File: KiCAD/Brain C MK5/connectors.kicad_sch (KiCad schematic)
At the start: 9 parts, among them J10 Conn_01x10, J3 Conn_01x06, J4 Conn_01x06, J6 Conn_01x10, J7 Conn_01x10, J8 Conn_01x04, J9 Conn_01x04

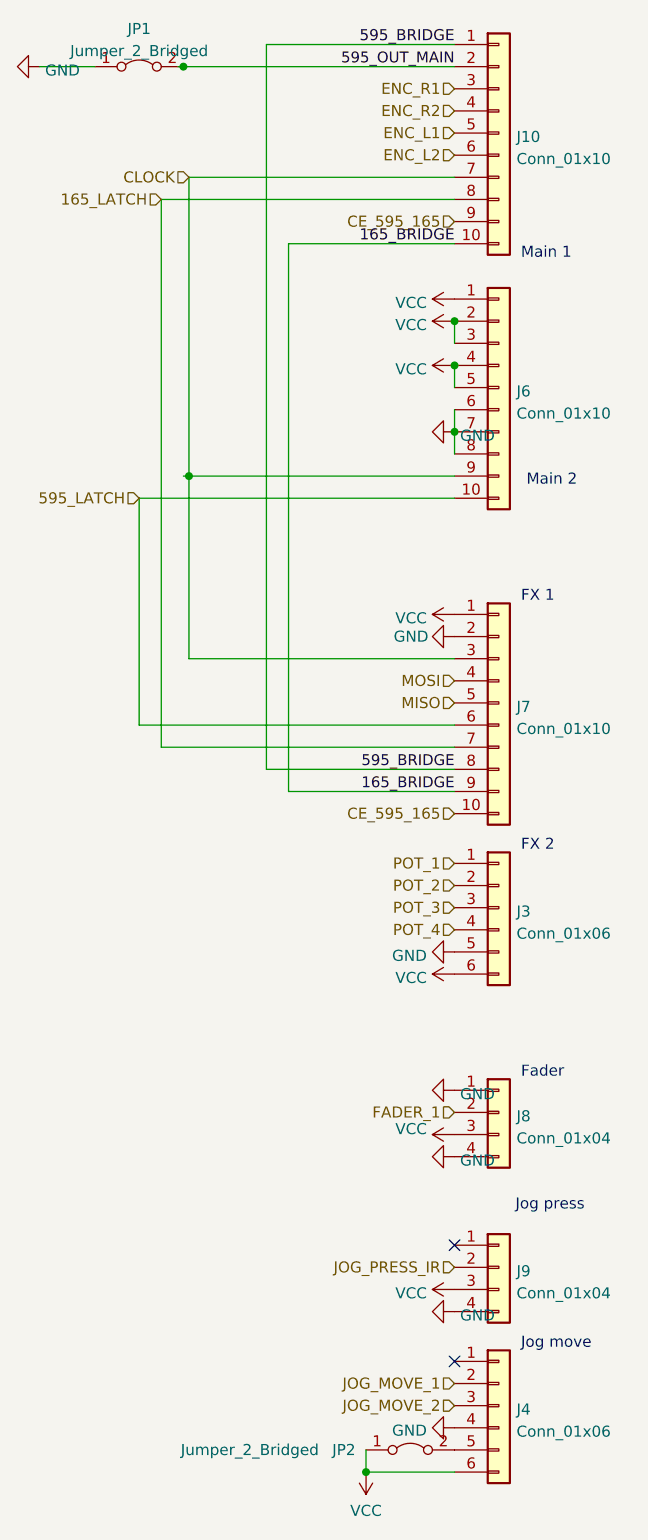
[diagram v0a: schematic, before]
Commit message: work
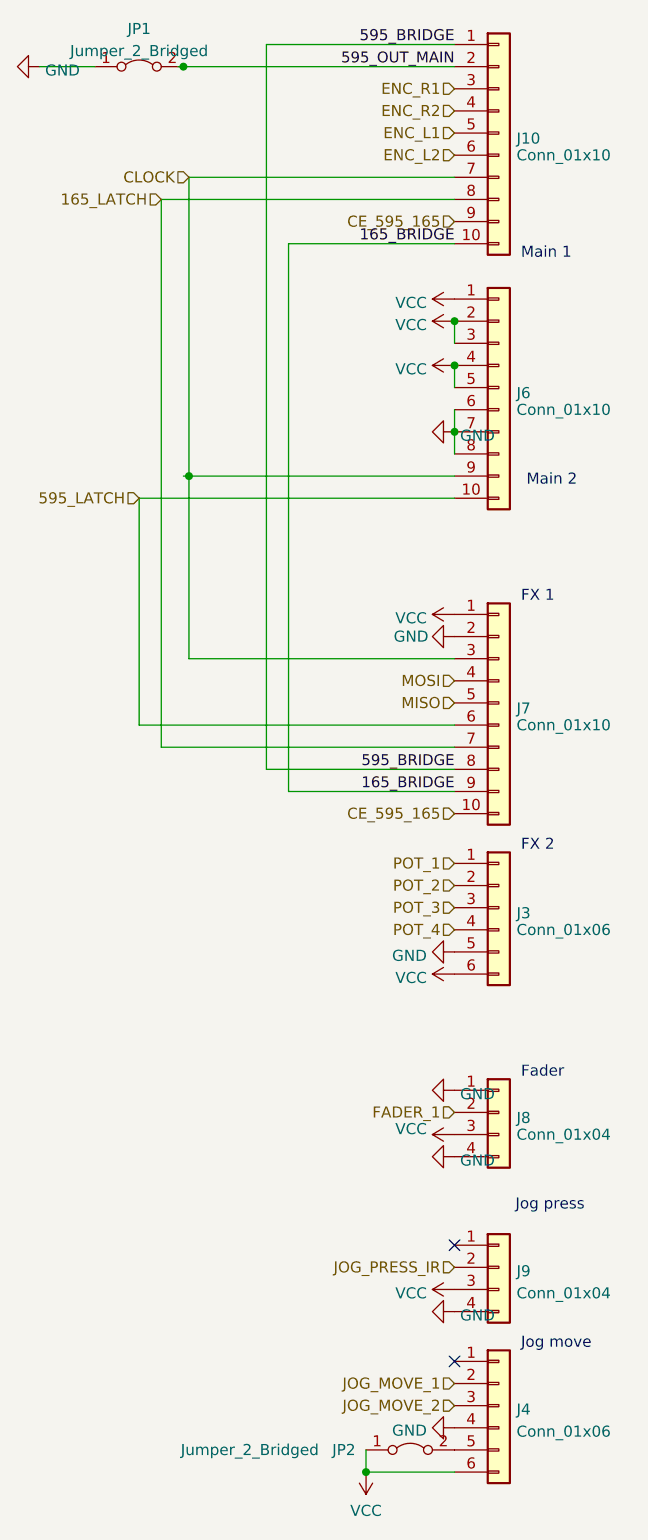
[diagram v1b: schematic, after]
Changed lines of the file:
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@@
   (symbol (lib_id "Connector_Generic:Conn_01x06") (at 278.13 113.03 0) (unit 1)
     (in_bom yes) (on_board yes) (dnp no) (fields_autoplaced)
-    (property "Reference" "J3" (at 280.162 113.4653 0)
-      (effects (font (size 1.27 1.27)) (justify left))
-    )
-    (property "Value" "Conn_01x06" (at 280.162 116.0022 0)
+    (property "Reference" "J3" (at 280.162 113.6563 0)
+      (effects (font (size 1.27 1.27)) (justify left))
+    )
+    (property "Value" "Conn_01x06" (at 280.162 115.5773 0)
       (effects (font (size 1.27 1.27)) (justify left))
     )
@@
         )
         (path "/0b6afff7-70c7-4317-8634-925834fa4d63/1ed31a1a-676b-43f1-be17-fc7627fd91ec"
-          (reference "J3") (unit 1)
+          (reference "J6") (unit 1)
         )
       )
@@
   (symbol (lib_id "Connector_Generic:Conn_01x10") (at 278.13 24.13 0) (unit 1)
     (in_bom yes) (on_board yes) (dnp no) (fields_autoplaced)
-    (property "Reference" "J10" (at 280.162 24.5653 0)
-      (effects (font (size 1.27 1.27)) (justify left))
-    )
-    (property "Value" "Conn_01x10" (at 280.162 27.1022 0)
+    (property "Reference" "J10" (at 280.162 24.7563 0)
+      (effects (font (size 1.27 1.27)) (justify left))
+    )
+    (property "Value" "Conn_01x10" (at 280.162 26.6773 0)
       (effects (font (size 1.27 1.27)) (justify left))
     )
@@
         )
         (path "/0b6afff7-70c7-4317-8634-925834fa4d63/1ed31a1a-676b-43f1-be17-fc7627fd91ec"
-          (reference "J9") (unit 1)
+          (reference "J3") (unit 1)
         )
       )
@@
   (symbol (lib_id "Connector_Generic:Conn_01x10") (at 278.13 53.34 0) (unit 1)
     (in_bom yes) (on_board yes) (dnp no) (fields_autoplaced)
-    (property "Reference" "J6" (at 280.162 53.7753 0)
-      (effects (font (size 1.27 1.27)) (justify left))
-    )
-    (property "Value" "Conn_01x10" (at 280.162 56.3122 0)
+    (property "Reference" "J6" (at 280.162 53.9663 0)
+      (effects (font (size 1.27 1.27)) (justify left))
+    )
+    (property "Value" "Conn_01x10" (at 280.162 55.8873 0)
       (effects (font (size 1.27 1.27)) (justify left))
     )
@@
         )
         (path "/0b6afff7-70c7-4317-8634-925834fa4d63/1ed31a1a-676b-43f1-be17-fc7627fd91ec"
-          (reference "J5") (unit 1)
+          (reference "J4") (unit 1)
         )
       )
@@
   (symbol (lib_id "Connector_Generic:Conn_01x04") (at 278.13 136.525 0) (unit 1)
     (in_bom yes) (on_board yes) (dnp no) (fields_autoplaced)
-    (property "Reference" "J8" (at 280.162 136.9603 0)
-      (effects (font (size 1.27 1.27)) (justify left))
-    )
-    (property "Value" "Conn_01x04" (at 280.162 139.4972 0)
+    (property "Reference" "J8" (at 280.162 137.1513 0)
+      (effects (font (size 1.27 1.27)) (justify left))
+    )
+    (property "Value" "Conn_01x04" (at 280.162 139.0723 0)
       (effects (font (size 1.27 1.27)) (justify left))
     )
@@
         )
         (path "/0b6afff7-70c7-4317-8634-925834fa4d63/1ed31a1a-676b-43f1-be17-fc7627fd91ec"
-          (reference "J4") (unit 1)
+          (reference "J9") (unit 1)
         )
       )
@@
   (symbol (lib_id "Connector_Generic:Conn_01x10") (at 278.13 89.535 0) (unit 1)
     (in_bom yes) (on_board yes) (dnp no) (fields_autoplaced)
-    (property "Reference" "J7" (at 280.162 89.9703 0)
-      (effects (font (size 1.27 1.27)) (justify left))
-    )
-    (property "Value" "Conn_01x10" (at 280.162 92.5072 0)
+    (property "Reference" "J7" (at 280.162 90.1613 0)
+      (effects (font (size 1.27 1.27)) (justify left))
+    )
+    (property "Value" "Conn_01x10" (at 280.162 92.0823 0)
       (effects (font (size 1.27 1.27)) (justify left))
     )
@@
         )
         (path "/0b6afff7-70c7-4317-8634-925834fa4d63/1ed31a1a-676b-43f1-be17-fc7627fd91ec"
-          (reference "J6") (unit 1)
-        )
-      )
+          (reference "J5") (unit 1)
+        )
+      )
